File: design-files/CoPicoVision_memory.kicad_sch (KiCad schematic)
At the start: 13 parts, among them U103 74ACT05, U201 GAL22V10, U202 GAL22V10, U203 AT28C64, U204 AS6C62256, U205 74HCT08, U206 74HCT74

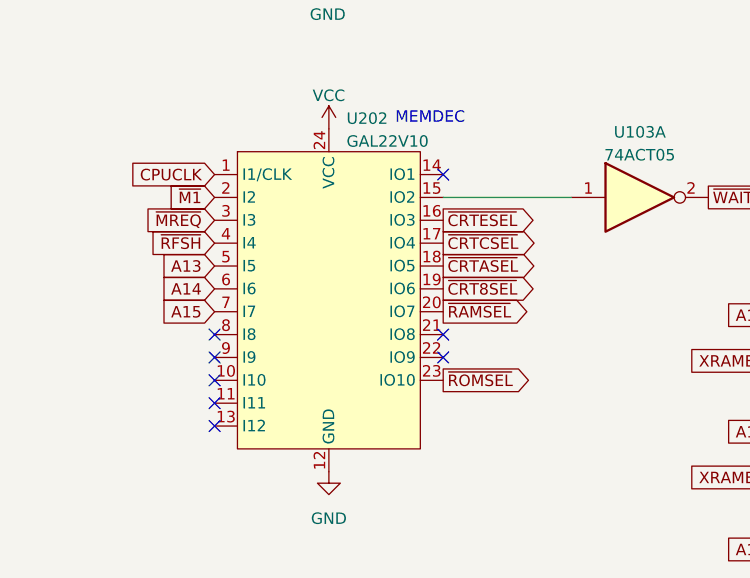
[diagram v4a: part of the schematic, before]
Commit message: Rearrange the MEMDEC GAL to work better with the new board layout.
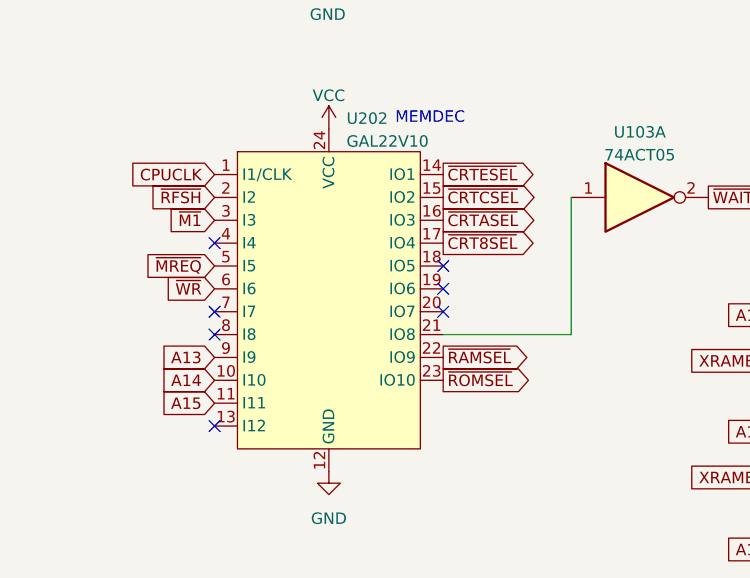
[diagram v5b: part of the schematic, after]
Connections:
- net A13: now also U202.9 (I9); no longer U202.5 (I5)
- net A14: now also U202.10 (I10); no longer U202.6 (I6)
- net A15: now also U202.11 (I11); no longer U202.7 (I7)
- net ~{CRT8SEL}: now also U202.17 (IO4); no longer U202.19 (IO6)
- net ~{CRTASEL}: now also U202.16 (IO3); no longer U202.18 (IO5)
- net ~{CRTCSEL}: now also U202.15 (IO2); no longer U202.17 (IO4)
- net ~{CRTESEL}: now also U202.14 (IO1); no longer U202.16 (IO3)
- net ~{M1}: now also U202.3 (I3); no longer U202.2 (I2)
- net ~{MREQ}: now also U202.5 (I5); no longer U202.3 (I3)
- net ~{RAMSEL}: now also U202.22 (IO9); no longer U202.20 (IO7)
- net ~{RFSH}: now also U202.2 (I2); no longer U202.4 (I4)
- net ~{WR}: now also U202.6 (I6)
- net at U103.1: now also U202.21 (IO8); no longer U202.15 (IO2)
- no-connect marks 16 -> 15
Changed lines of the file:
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@@
   (junction (at 99.441 155.956) (diameter 0) (color 0 0 0 0)
   )
-  (no_connect (at 95.885 124.079))
-  (no_connect (at 121.285 121.539))
-  (no_connect (at 121.285 103.759))
-  (no_connect (at 95.885 129.159))
   (no_connect (at 121.158 47.752))
   (no_connect (at 95.885 131.699))
   (no_connect (at 95.758 52.832))
-  (no_connect (at 95.885 126.619))
+  (no_connect (at 121.285 113.919))
   (no_connect (at 95.758 75.692))
   (no_connect (at 121.158 50.292))
   (no_connect (at 95.885 121.539))
   (no_connect (at 161.925 32.258))
-  (no_connect (at 121.285 124.079))
+  (no_connect (at 95.885 118.999))
+  (no_connect (at 121.285 118.999))
+  (no_connect (at 121.285 116.459))
   (no_connect (at 121.158 52.832))
   (no_connect (at 161.925 59.309))
+  (no_connect (at 95.885 111.379))
   (no_connect (at 173.863 161.671))
   (wire (pts (xy 154.305 42.164) (xy 154.305 37.338))
@@
     (stroke (width 0) (type default))
   )
+  (wire (pts (xy 135.509 106.299) (xy 135.509 121.539))
+    (stroke (width 0) (type default))
+  )
   (wire (pts (xy 121.412 166.497) (xy 121.412 163.957))
     (stroke (width 0) (type default))
@@
     (stroke (width 0) (type default))
   )
+  (wire (pts (xy 135.509 121.539) (xy 121.285 121.539))
+    (stroke (width 0) (type default))
+  )
   (wire (pts (xy 99.441 161.036) (xy 110.871 161.036))
     (stroke (width 0) (type default))
@@
   )
   (wire (pts (xy 99.441 155.956) (xy 110.871 155.956))
-    (stroke (width 0) (type default))
-  )
-  (wire (pts (xy 121.285 106.299) (xy 135.509 106.299))
     (stroke (width 0) (type default))
   )
@@
     )
   )
-  (global_label "~{RAMSEL}" (shape output) (at 121.285 118.999 0) (fields_autoplaced)
-    (effects (font (size 1.27 1.27)) (justify left))
-    (property "Intersheetrefs" "${INTERSHEET_REFS}" (at 131.3874 118.999 0)
+  (global_label "~{RAMSEL}" (shape output) (at 121.285 124.079 0) (fields_autoplaced)
+    (effects (font (size 1.27 1.27)) (justify left))
+    (property "Intersheetrefs" "${INTERSHEET_REFS}" (at 131.3874 124.079 0)
       (effects (font (size 1.27 1.27)) (justify left) hide)
     )
@@
     )
   )
-  (global_label "~{CRTASEL}" (shape output) (at 121.285 113.919 0) (fields_autoplaced)
-    (effects (font (size 1.27 1.27)) (justify left))
-    (property "Intersheetrefs" "${INTERSHEET_REFS}" (at 132.1736 113.919 0)
+  (global_label "~{CRTASEL}" (shape output) (at 121.285 108.839 0) (fields_autoplaced)
+    (effects (font (size 1.27 1.27)) (justify left))
+    (property "Intersheetrefs" "${INTERSHEET_REFS}" (at 132.1736 108.839 0)
       (effects (font (size 1.27 1.27)) (justify left) hide)
     )
@@
     )
   )
-  (global_label "A13" (shape input) (at 95.885 113.919 180) (fields_autoplaced)
-    (effects (font (size 1.27 1.27)) (justify right))
-    (property "Intersheetrefs" "${INTERSHEET_REFS}" (at 89.4716 113.919 0)
+  (global_label "A13" (shape input) (at 95.885 124.079 180) (fields_autoplaced)
+    (effects (font (size 1.27 1.27)) (justify right))
+    (property "Intersheetrefs" "${INTERSHEET_REFS}" (at 89.4716 124.079 0)
       (effects (font (size 1.27 1.27)) (justify right) hide)
     )
@@
     )
   )
-  (global_label "~{M1}" (shape input) (at 95.885 106.299 180) (fields_autoplaced)
-    (effects (font (size 1.27 1.27)) (justify right))
-    (property "Intersheetrefs" "${INTERSHEET_REFS}" (at 90.3183 106.299 0)
+  (global_label "~{M1}" (shape input) (at 95.885 108.839 180) (fields_autoplaced)
+    (effects (font (size 1.27 1.27)) (justify right))
+    (property "Intersheetrefs" "${INTERSHEET_REFS}" (at 90.3183 108.839 0)
       (effects (font (size 1.27 1.27)) (justify right) hide)
     )
@@
     )
   )
-  (global_label "A14" (shape input) (at 95.885 116.459 180) (fields_autoplaced)
-    (effects (font (size 1.27 1.27)) (justify right))
-    (property "Intersheetrefs" "${INTERSHEET_REFS}" (at 89.4716 116.459 0)
+  (global_label "A14" (shape input) (at 95.885 126.619 180) (fields_autoplaced)
+    (effects (font (size 1.27 1.27)) (justify right))
+    (property "Intersheetrefs" "${INTERSHEET_REFS}" (at 89.4716 126.619 0)
       (effects (font (size 1.27 1.27)) (justify right) hide)
     )
@@
     )
   )
+  (global_label "~{WR}" (shape input) (at 95.885 116.459 180) (fields_autoplaced)
+    (effects (font (size 1.27 1.27)) (justify right))
+    (property "Intersheetrefs" "${INTERSHEET_REFS}" (at 90.2578 116.459 0)
+      (effects (font (size 1.27 1.27)) (justify right) hide)
+    )
+  )
   (global_label "A7" (shape input) (at 95.758 55.372 180) (fields_autoplaced)
     (effects (font (size 1.27 1.27)) (justify right))
@@
     )
   )
-  (global_label "~{CRTESEL}" (shape output) (at 121.285 108.839 0) (fields_autoplaced)
-    (effects (font (size 1.27 1.27)) (justify left))
-    (property "Intersheetrefs" "${INTERSHEET_REFS}" (at 132.234 108.839 0)
+  (global_label "~{CRTESEL}" (shape output) (at 121.285 103.759 0) (fields_autoplaced)
+    (effects (font (size 1.27 1.27)) (justify left))
+    (property "Intersheetrefs" "${INTERSHEET_REFS}" (at 132.234 103.759 0)
       (effects (font (size 1.27 1.27)) (justify left) hide)
     )
@@
     )
   )
-  (global_label "~{CRTCSEL}" (shape output) (at 121.285 111.379 0) (fields_autoplaced)
-    (effects (font (size 1.27 1.27)) (justify left))
-    (property "Intersheetrefs" "${INTERSHEET_REFS}" (at 132.355 111.379 0)
-      (effects (font (size 1.27 1.27)) (justify left) hide)
-    )
-  )
-  (global_label "~{RFSH}" (shape input) (at 95.885 111.379 180) (fields_autoplaced)
-    (effects (font (size 1.27 1.27)) (justify right))
-    (property "Intersheetrefs" "${INTERSHEET_REFS}" (at 88.0806 111.379 0)
-      (effects (font (size 1.27 1.27)) (justify right) hide)
-    )
-  )
-  (global_label "A15" (shape input) (at 95.885 118.999 180) (fields_autoplaced)
-    (effects (font (size 1.27 1.27)) (justify right))
-    (property "Intersheetrefs" "${INTERSHEET_REFS}" (at 89.4716 118.999 0)
+  (global_label "~{CRTCSEL}" (shape output) (at 121.285 106.299 0) (fields_autoplaced)
+    (effects (font (size 1.27 1.27)) (justify left))
+    (property "Intersheetrefs" "${INTERSHEET_REFS}" (at 132.355 106.299 0)
+      (effects (font (size 1.27 1.27)) (justify left) hide)
+    )
+  )
+  (global_label "~{RFSH}" (shape input) (at 95.885 106.299 180) (fields_autoplaced)
+    (effects (font (size 1.27 1.27)) (justify right))
+    (property "Intersheetrefs" "${INTERSHEET_REFS}" (at 88.0806 106.299 0)
+      (effects (font (size 1.27 1.27)) (justify right) hide)
+    )
+  )
+  (global_label "A15" (shape input) (at 95.885 129.159 180) (fields_autoplaced)
+    (effects (font (size 1.27 1.27)) (justify right))
+    (property "Intersheetrefs" "${INTERSHEET_REFS}" (at 89.4716 129.159 0)
       (effects (font (size 1.27 1.27)) (justify right) hide)
     )
@@
     )
   )
-  (global_label "~{MREQ}" (shape input) (at 95.885 108.839 180) (fields_autoplaced)
-    (effects (font (size 1.27 1.27)) (justify right))
-    (property "Intersheetrefs" "${INTERSHEET_REFS}" (at 87.7783 108.839 0)
-      (effects (font (size 1.27 1.27)) (justify right) hide)
-    )
-  )
-  (global_label "~{CRT8SEL}" (shape output) (at 121.285 116.459 0) (fields_autoplaced)
-    (effects (font (size 1.27 1.27)) (justify left))
-    (property "Intersheetrefs" "${INTERSHEET_REFS}" (at 132.2945 116.459 0)
-      (effects (font (size 1.27 1.27)) (justify left) hide)
-    )
+  (global_label "~{MREQ}" (shape input) (at 95.885 113.919 180) (fields_autoplaced)
+    (effects (font (size 1.27 1.27)) (justify right))
+    (property "Intersheetrefs" "${INTERSHEET_REFS}" (at 87.7783 113.919 0)
+      (effects (font (size 1.27 1.27)) (justify right) hide)
+    )
+  )
+  (global_label "~{CRT8SEL}" (shape output) (at 121.285 111.379 0) (fields_autoplaced)
+    (effects (font (size 1.27 1.27)) (justify left))
+    (property "Intersheetrefs" "${INTERSHEET_REFS}" (at 132.2945 111.379 0)
+      (effects (font (size 1.27 1.27)) (justify left) hide)
+    )

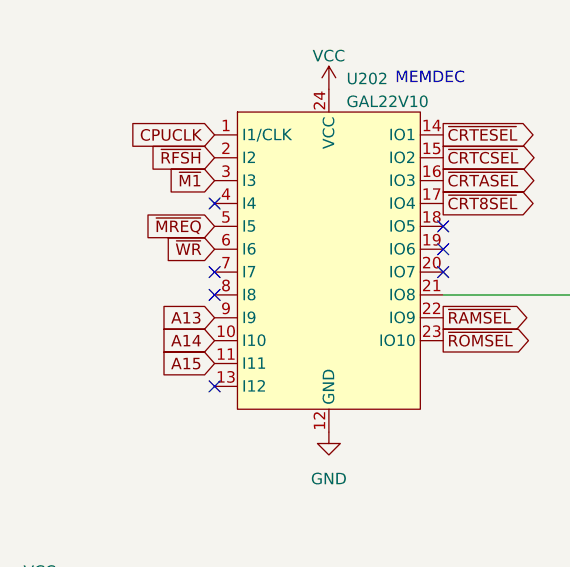
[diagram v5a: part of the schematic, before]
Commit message: Add the XRAMEN and ROMEN signals to the MEMDEC GAL.
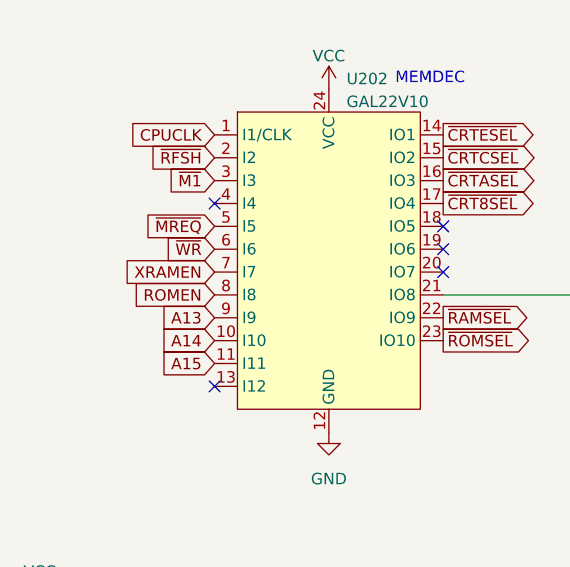
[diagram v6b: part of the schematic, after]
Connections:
- net ROMEN: now also U202.8 (I8)
- net XRAMEN: now also U202.7 (I7)
- no-connect marks 15 -> 13
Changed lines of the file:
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@@
   (no_connect (at 95.758 75.692))
   (no_connect (at 121.158 50.292))
-  (no_connect (at 95.885 121.539))
   (no_connect (at 161.925 32.258))
-  (no_connect (at 95.885 118.999))
   (no_connect (at 121.285 118.999))
   (no_connect (at 121.285 116.459))
@@
     )
   )
+  (global_label "XRAMEN" (shape input) (at 95.885 118.999 180) (fields_autoplaced)
+    (effects (font (size 1.27 1.27)) (justify right))
+    (property "Intersheetrefs" "${INTERSHEET_REFS}" (at 85.4802 118.999 0)
+      (effects (font (size 1.27 1.27)) (justify right) hide)
+    )
+  )
   (global_label "D6" (shape bidirectional) (at 213.995 116.84 0) (fields_autoplaced)
     (effects (font (size 1.27 1.27)) (justify left))
@@
       (effects (font (size 1.27 1.27)) (justify right) hide)
     )
+  )
+  (global_label "ROMEN" (shape input) (at 95.885 121.539 180) (fields_autoplaced)
+    (effects (font (size 1.27 1.27)) (justify right))
+    (property "Intersheetrefs" "${INTERSHEET_REFS}" (at 86.4478 121.539 0)
+      (effects (font (size 1.27 1.27)) (justify right) hide)
+    )

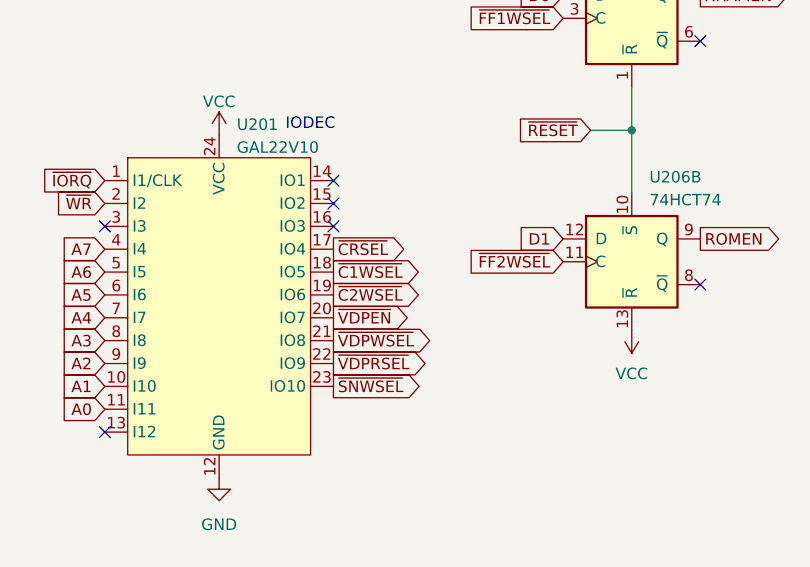
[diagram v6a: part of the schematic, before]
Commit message: Add all of the SGM IODEC signals and re-pin the outputs to work better with the new board layout.
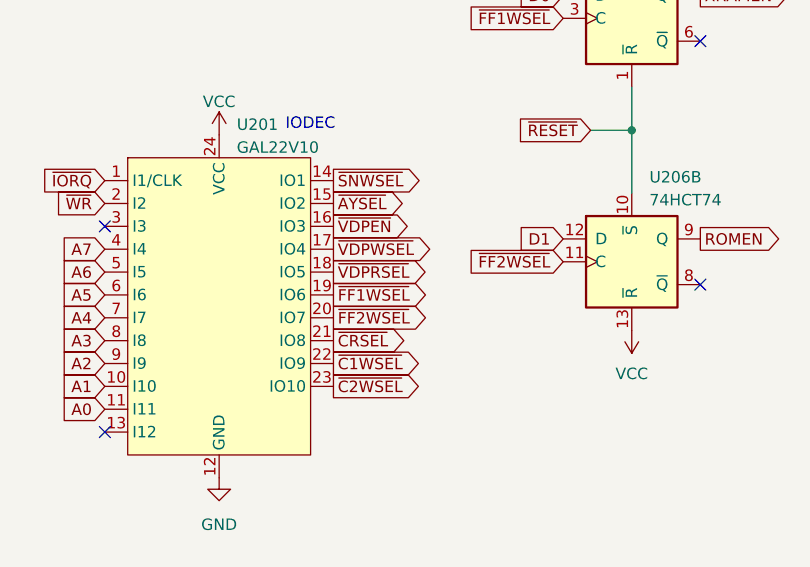
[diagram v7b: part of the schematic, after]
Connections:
- net ~{C1WSEL}: now also U201.22 (IO9); no longer U201.18 (IO5)
- net ~{C2WSEL}: now also U201.23 (IO10); no longer U201.19 (IO6)
- net ~{CRSEL}: now also U201.21 (IO8); no longer U201.17 (IO4)
- net ~{FF1WSEL}: now also U201.19 (IO6)
- net ~{FF2WSEL}: now also U201.20 (IO7)
- net ~{SNWSEL}: now also U201.14 (IO1); no longer U201.23 (IO10)
- net ~{VDPEN}: now also U201.16 (IO3); no longer U201.20 (IO7)
- net ~{VDPRSEL}: now also U201.18 (IO5); no longer U201.22 (IO9)
- net ~{VDPWSEL}: now also U201.17 (IO4); no longer U201.21 (IO8)
- net ~{AYSEL}: now reaches U201.15 (IO2)
- no-connect marks 13 -> 10
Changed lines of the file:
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@@
   (junction (at 99.441 155.956) (diameter 0) (color 0 0 0 0)
   )
-  (no_connect (at 121.158 47.752))
   (no_connect (at 95.885 131.699))
   (no_connect (at 95.758 52.832))
   (no_connect (at 121.285 113.919))
   (no_connect (at 95.758 75.692))
-  (no_connect (at 121.158 50.292))
   (no_connect (at 161.925 32.258))
   (no_connect (at 121.285 118.999))
   (no_connect (at 121.285 116.459))
-  (no_connect (at 121.158 52.832))
   (no_connect (at 161.925 59.309))
   (no_connect (at 95.885 111.379))
@@
     )
   )
-  (global_label "~{VDPWSEL}" (shape output) (at 121.158 65.532 0) (fields_autoplaced)
-    (effects (font (size 1.27 1.27)) (justify left))
-    (property "Intersheetrefs" "${INTERSHEET_REFS}" (at 132.5304 65.532 0)
+  (global_label "~{VDPWSEL}" (shape output) (at 121.158 55.372 0) (fields_autoplaced)
+    (effects (font (size 1.27 1.27)) (justify left))
+    (property "Intersheetrefs" "${INTERSHEET_REFS}" (at 132.5304 55.372 0)
       (effects (font (size 1.27 1.27)) (justify left) hide)
     )
@@
     )
   )
-  (global_label "~{C1WSEL}" (shape output) (at 121.158 57.912 0) (fields_autoplaced)
-    (effects (font (size 1.27 1.27)) (justify left))
-    (property "Intersheetrefs" "${INTERSHEET_REFS}" (at 131.3813 57.912 0)
+  (global_label "~{C1WSEL}" (shape output) (at 121.158 68.072 0) (fields_autoplaced)
+    (effects (font (size 1.27 1.27)) (justify left))
+    (property "Intersheetrefs" "${INTERSHEET_REFS}" (at 131.3813 68.072 0)
       (effects (font (size 1.27 1.27)) (justify left) hide)
     )
@@
     )
   )
-  (global_label "~{CRSEL}" (shape output) (at 121.158 55.372 0) (fields_autoplaced)
-    (effects (font (size 1.27 1.27)) (justify left))
-    (property "Intersheetrefs" "${INTERSHEET_REFS}" (at 129.9904 55.372 0)
+  (global_label "~{CRSEL}" (shape output) (at 121.158 65.532 0) (fields_autoplaced)
+    (effects (font (size 1.27 1.27)) (justify left))
+    (property "Intersheetrefs" "${INTERSHEET_REFS}" (at 129.9904 65.532 0)
       (effects (font (size 1.27 1.27)) (justify left) hide)
     )
@@
     )
   )
-  (global_label "~{VDPEN}" (shape output) (at 121.158 62.992 0) (fields_autoplaced)
-    (effects (font (size 1.27 1.27)) (justify left))
-    (property "Intersheetrefs" "${INTERSHEET_REFS}" (at 130.1719 62.992 0)
+  (global_label "~{VDPEN}" (shape output) (at 121.158 52.832 0) (fields_autoplaced)
+    (effects (font (size 1.27 1.27)) (justify left))
+    (property "Intersheetrefs" "${INTERSHEET_REFS}" (at 130.1719 52.832 0)
       (effects (font (size 1.27 1.27)) (justify left) hide)
     )
@@
     )
   )
+  (global_label "~{FF2WSEL}" (shape output) (at 121.158 62.992 0) (fields_autoplaced)
+    (effects (font (size 1.27 1.27)) (justify left))
+    (property "Intersheetrefs" "${INTERSHEET_REFS}" (at 132.2885 62.992 0)
+      (effects (font (size 1.27 1.27)) (justify left) hide)
+    )
+  )
   (global_label "A2" (shape input) (at 95.758 68.072 180) (fields_autoplaced)
     (effects (font (size 1.27 1.27)) (justify right))
@@
     )
   )
+  (global_label "~{FF1WSEL}" (shape output) (at 121.158 60.452 0) (fields_autoplaced)
+    (effects (font (size 1.27 1.27)) (justify left))
+    (property "Intersheetrefs" "${INTERSHEET_REFS}" (at 132.2885 60.452 0)
+      (effects (font (size 1.27 1.27)) (justify left) hide)
+    )
+  )
   (global_label "D6" (shape bidirectional) (at 213.995 116.84 0) (fields_autoplaced)
     (effects (font (size 1.27 1.27)) (justify left))
@@
     )
   )
-  (global_label "~{SNWSEL}" (shape output) (at 121.158 70.612 0) (fields_autoplaced)
-    (effects (font (size 1.27 1.27)) (justify left))
-    (property "Intersheetrefs" "${INTERSHEET_REFS}" (at 131.4418 70.612 0)
+  (global_label "~{SNWSEL}" (shape output) (at 121.158 47.752 0) (fields_autoplaced)
+    (effects (font (size 1.27 1.27)) (justify left))
+    (property "Intersheetrefs" "${INTERSHEET_REFS}" (at 131.4418 47.752 0)
       (effects (font (size 1.27 1.27)) (justify left) hide)
     )
@@
     )
   )
-  (global_label "~{C2WSEL}" (shape output) (at 121.158 60.452 0) (fields_autoplaced)
-    (effects (font (size 1.27 1.27)) (justify left))
-    (property "Intersheetrefs" "${INTERSHEET_REFS}" (at 131.3813 60.452 0)
+  (global_label "~{C2WSEL}" (shape output) (at 121.158 70.612 0) (fields_autoplaced)
+    (effects (font (size 1.27 1.27)) (justify left))
+    (property "Intersheetrefs" "${INTERSHEET_REFS}" (at 131.3813 70.612 0)
       (effects (font (size 1.27 1.27)) (justify left) hide)
     )
@@
     )
   )
-  (global_label "~{VDPRSEL}" (shape output) (at 121.158 68.072 0) (fields_autoplaced)
-    (effects (font (size 1.27 1.27)) (justify left))
-    (property "Intersheetrefs" "${INTERSHEET_REFS}" (at 132.349 68.072 0)
+  (global_label "~{VDPRSEL}" (shape output) (at 121.158 57.912 0) (fields_autoplaced)
+    (effects (font (size 1.27 1.27)) (justify left))
+    (property "Intersheetrefs" "${INTERSHEET_REFS}" (at 132.349 57.912 0)
       (effects (font (size 1.27 1.27)) (justify left) hide)
     )
@@
       (effects (font (size 1.27 1.27)) (justify left) hide)
     )
+  )
+  (global_label "~{AYSEL}" (shape output) (at 121.158 50.292 0) (fields_autoplaced)
+    (effects (font (size 1.27 1.27)) (justify left))
+    (property "Intersheetrefs" "${INTERSHEET_REFS}" (at 129.6276 50.292 0)
+      (effects (font (size 1.27 1.27)) (justify left) hide)
+    )
